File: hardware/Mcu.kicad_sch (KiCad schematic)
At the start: 22 parts, among them U1 STM32G484RETx, Y1 X322516MLB4SI, Y2 Q13FC1350000400

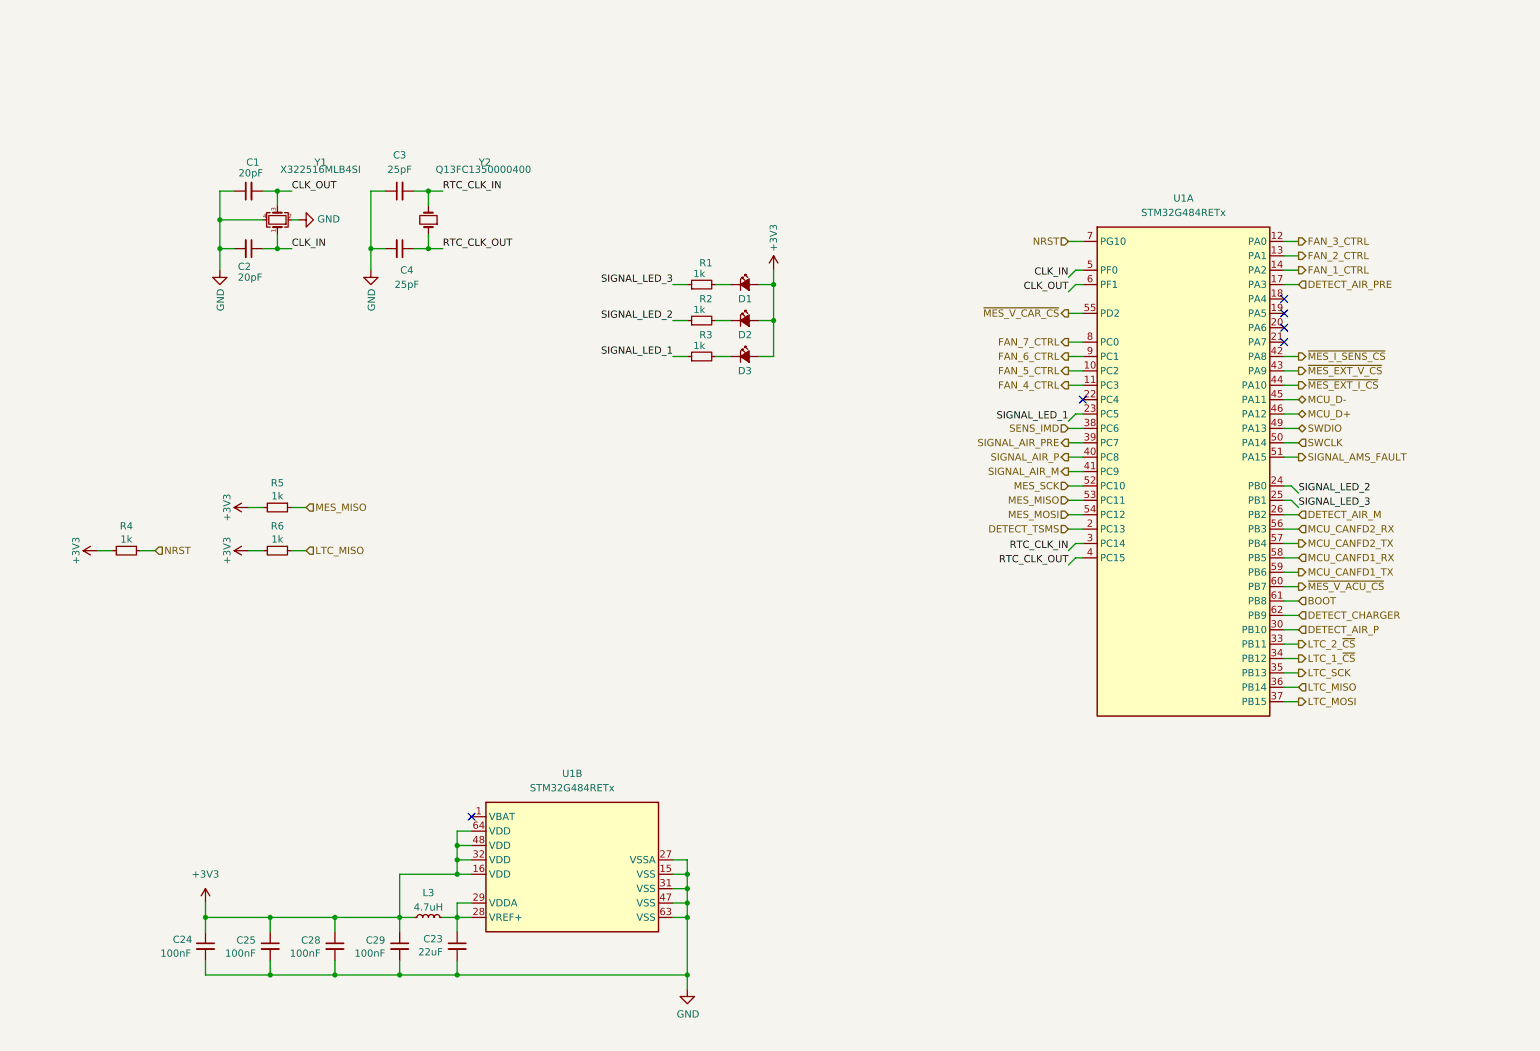
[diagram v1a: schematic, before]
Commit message: sync
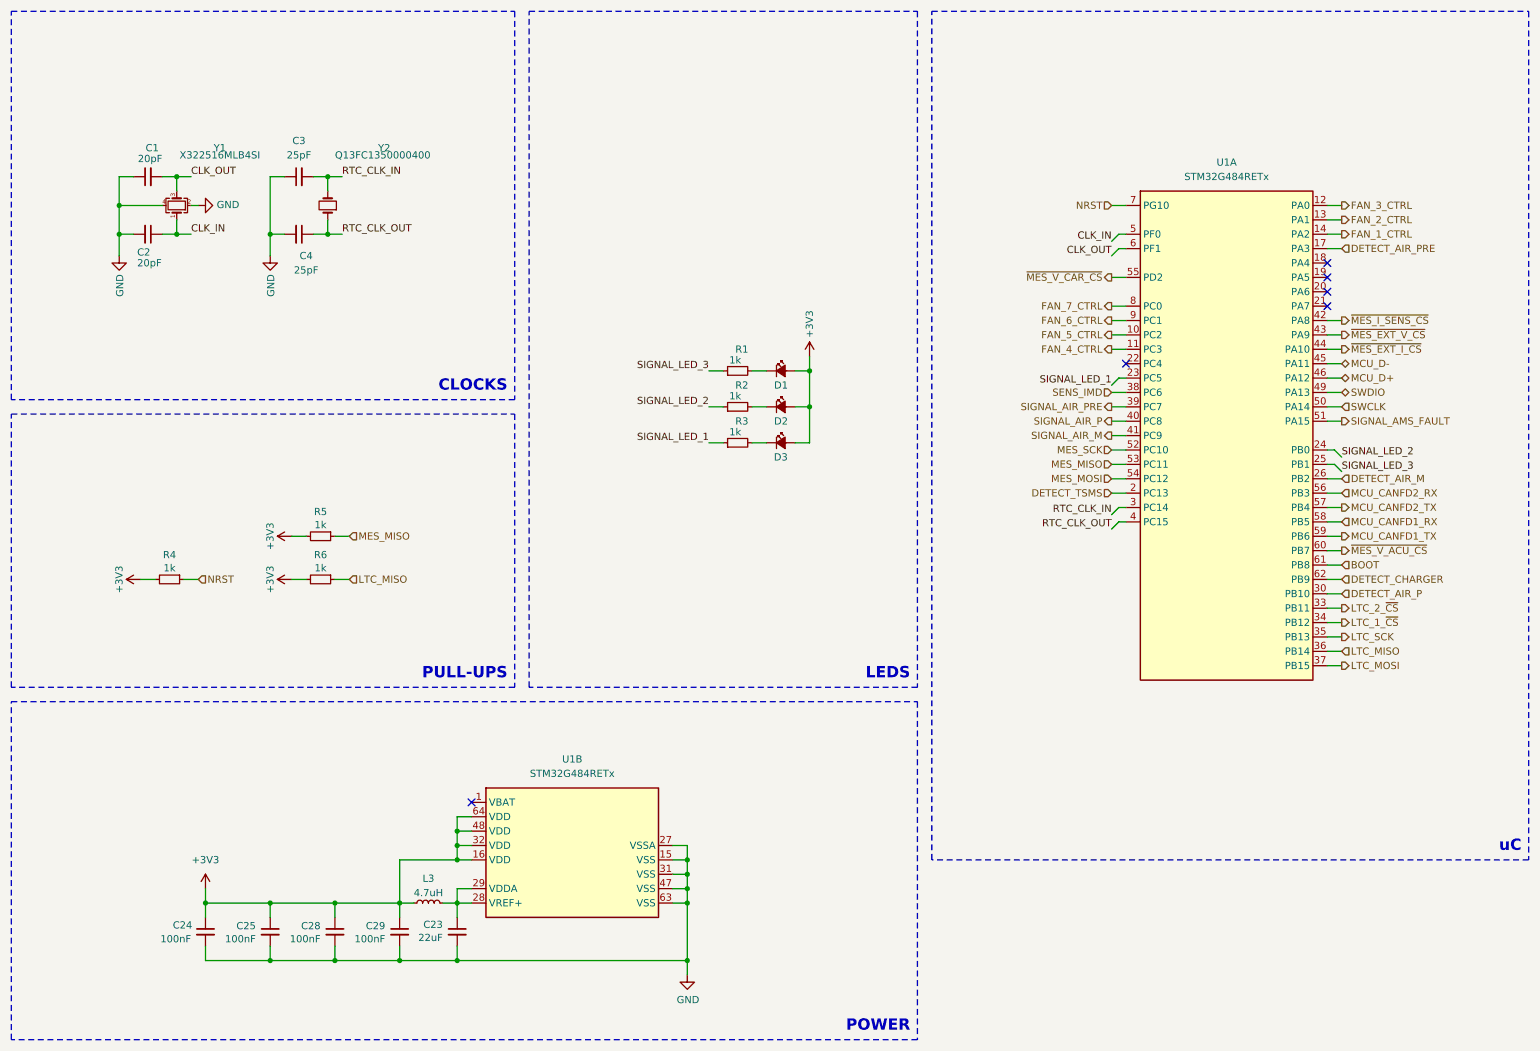
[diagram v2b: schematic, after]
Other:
- note added: "CLOCKS"
- note added: "LEDS"
- note added: "POWER"
- note added: "PULL-UPS"
- note added: "uC"
- moved on the sheet: C1, C2, C23, C24, C25, C28, C29, C3, C4, D1, D2, D3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
